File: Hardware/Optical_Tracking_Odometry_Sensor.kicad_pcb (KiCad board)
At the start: 2 copper layers, 25.4 x 25.4 mm, 55 parts, among them J3 CONN_06NO_SILK_NO_POP, Q1 100mA/20V/3.8Ω, Q2 100mA/20V/3.8Ω, U1 PAA5160E1-Q, U2 LSM6DS0, U3 STM32C011F6U6, U4 RT9080-18GJ5

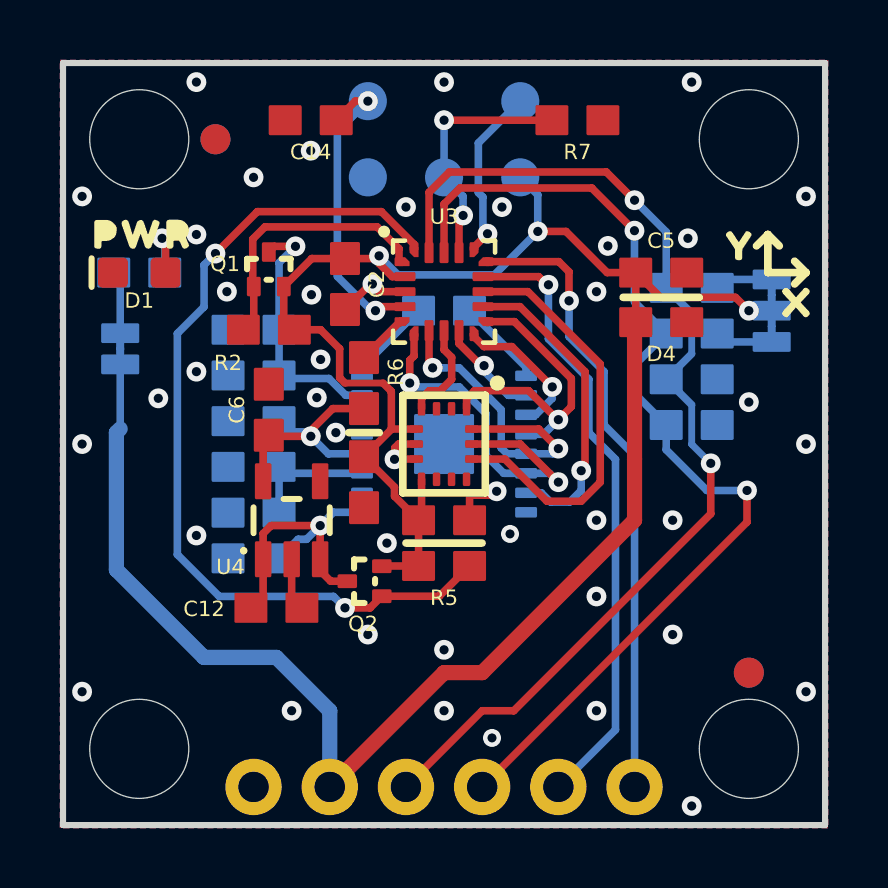
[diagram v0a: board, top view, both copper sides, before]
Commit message: yepyep
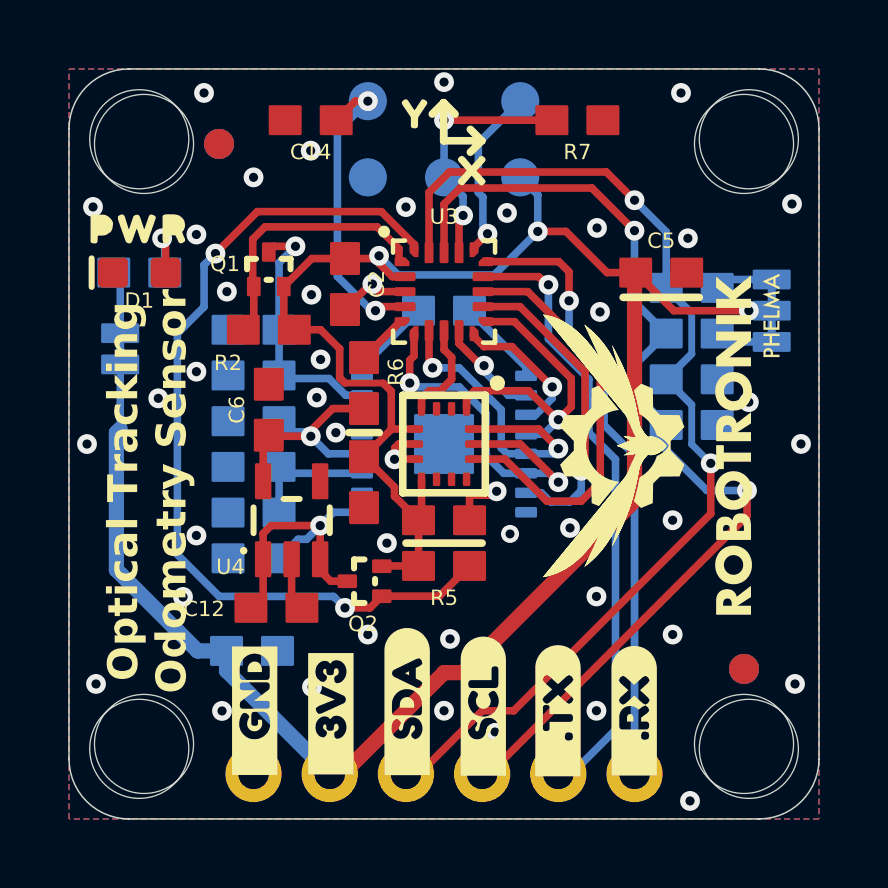
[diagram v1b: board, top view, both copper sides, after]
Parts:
- removed U$20: , Optical_Tracking_Odometry_Sensor:#PWR#0
- removed U$21: , Optical_Tracking_Odometry_Sensor:TOUCH##0
- removed U$22: , Optical_Tracking_Odometry_Sensor:DO_NOT0
- removed U$26: , Optical_Tracking_Odometry_Sensor:#I2C#0
- removed U$28: , Optical_Tracking_Odometry_Sensor:850NM0
- removed U$6: , Optical_Tracking_Odometry_Sensor:CLASS_1_LASER0
- added ?: , , F.Cu at (158.5, 95.0)
- added ?: , , F.Cu at (158.5, 115.0)
- added ?: , , F.Cu at (138.5, 95.0)
- added H1: STAND-OFF, Optical_Tracking_Odometry_Sensor:STAND-OFF, F.Cu at (138.5, 115.0)
- added kibuzzard-68FE4977: G***, kibuzzard-68FE4977, B.Cu at (159.4, 103.9)
- added kibuzzard-68FE49AD: G***, kibuzzard-68FE49AD, B.Cu at (137.7, 105.1)
- added kibuzzard-68FE4A6E: G***, kibuzzard-68FE4A6E, F.Cu at (142.2, 113.9)
- added kibuzzard-68FE4A91: G***, kibuzzard-68FE4A91, F.Cu at (144.7, 114.0)
- added kibuzzard-68FE4AB9: G***, kibuzzard-68FE4AB9, F.Cu at (147.3, 113.6)
- added kibuzzard-68FE4AC0: G***, kibuzzard-68FE4AC0, F.Cu at (149.8, 113.7)
- added kibuzzard-68FE4B1F: G***, kibuzzard-68FE4B1F, F.Cu at (152.3, 113.9)
- added kibuzzard-68FE4B2A: G***, kibuzzard-68FE4B2A, F.Cu at (154.8, 113.9)
- D4: moved to B.Cu
- moved D4 17.5 mm to (142.1, 111.9)
- moved U$29 11.7 mm to (147.6, 94.0)
- moved U$18 11.7 mm to (149.5, 95.9)
- moved J3 0.43 mm to (142.2, 116.0)
- moved U$25 0.22 mm to (138.3, 97.8)
- moved FD3 0.20 mm to (158.5, 112.5)
- moved FD4 0.20 mm to (158.5, 112.5)
- moved FD1 0.20 mm to (141.0, 95.0)
- moved FD2 0.20 mm to (141.0, 95.0)
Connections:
- net 3.3V renamed +3.3V
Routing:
- net +3.3V: track 79.3 -> 77.6 mm
- net GND: vias 42 -> 44
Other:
- board size 25.4 x 25.4 mm -> 25 x 25 mm
- board text added: "Class 1 Laser 850nm"
- board text added: "DO NOT TOUCH!"
- board text added: "Optical Tracking Odometry Sensor"
